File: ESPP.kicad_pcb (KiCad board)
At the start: 2 copper layers, 18 parts, among them P1 USB_OTG, Q1 MMBT3904, Q2 MMBT3904, U1 RT9193, U2 CH340G, X1 12MHz, X2 ESP-PROG

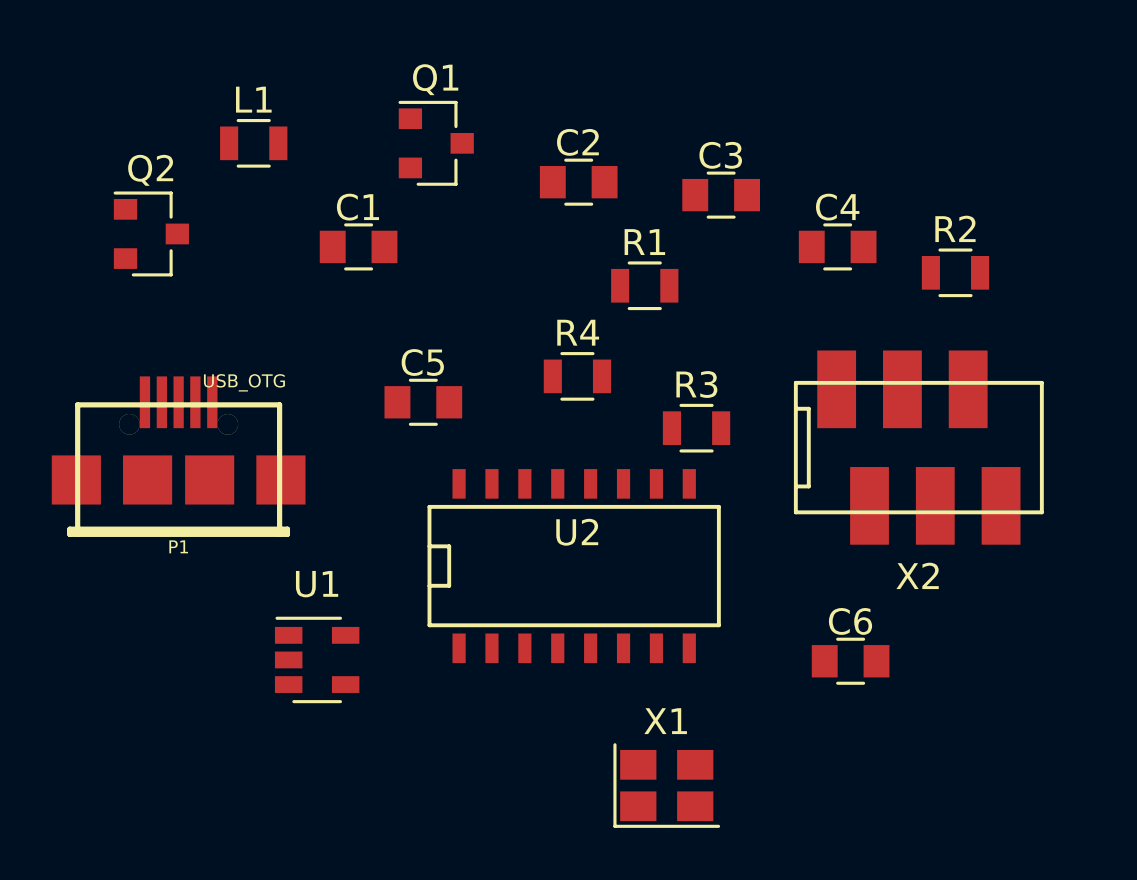
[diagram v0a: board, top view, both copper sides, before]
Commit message: WIP
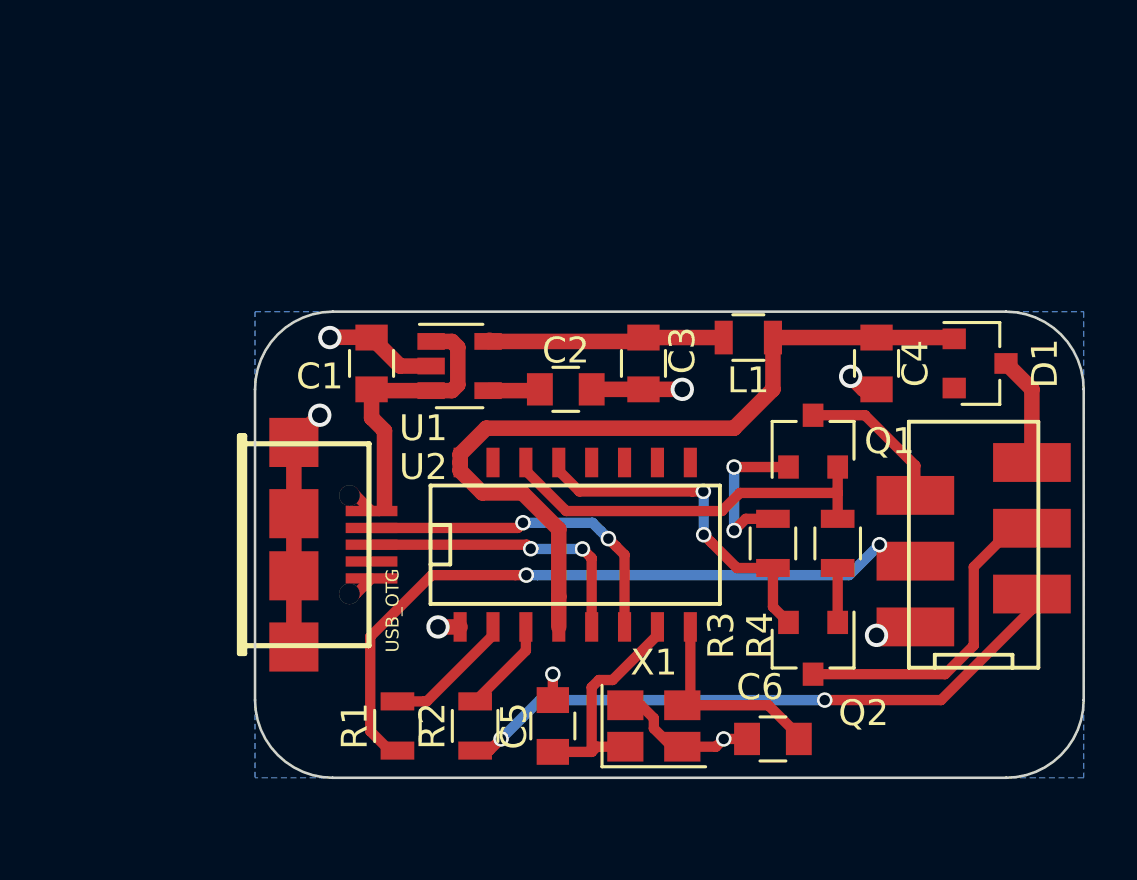
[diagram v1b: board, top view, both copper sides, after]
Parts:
- added D1: BAT54C, TO_SOT_Packages_SMD:SOT-23, F.Cu at (163.0, 105.0)
- added REF***: OSHW-Logo_11.4x12mm_SilkScreen, Symbols:OSHW-Logo_11.4x12mm_SilkScreen, B.Cu at (152.5, 112.0)
- C3: value 47u -> 1u
- moved Q2 30.1 mm to (156.6, 116.0), turned to 270 degrees
- moved R2 25.5 mm to (143.5, 119.0), turned to 90 degrees
- moved L1 20.5 mm to (154.1, 104.0), turned to 180 degrees
- moved R1 19.5 mm to (140.5, 119.0), turned to 90 degrees
- moved Q1 18.5 mm to (156.6, 108.0), turned to 90 degrees
- moved C5 13.5 mm to (146.5, 119.0), turned to 90 degrees
- moved U1 12.6 mm to (142.9, 105.1)
- moved R4 11.9 mm to (157.5, 112.0), turned to 90 degrees
- moved C2 8.02 mm to (147.0, 106.0)
- moved C3 7.16 mm to (150.0, 105.0), turned to 270 degrees
- moved R3 5.34 mm to (155.0, 112.0), turned to 90 degrees
- moved P1 5.10 mm to (136.5, 112.0), turned to 270 degrees
- moved C4 4.74 mm to (159.0, 105.0), turned to 270 degrees
- moved C1 4.53 mm to (139.5, 105.0), turned to 90 degrees
- moved X2 4.31 mm to (162.8, 112.0), turned to 90 degrees
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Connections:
- net /5V renamed /5V-USB
- X2 pad 6: VCC -> Net-(D1-Pad3)
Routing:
- net VCC: track 0.00 -> 31.3 mm
- net GND: track 0.00 -> 28.9 mm, vias 0 -> 8
- net /RX: track 0.00 -> 28.3 mm, vias 0 -> 2
- net /TX: track 0.00 -> 24.3 mm, vias 0 -> 2
- net /RTS: track 0.00 -> 15.3 mm
- net /DTR: track 0.00 -> 13.5 mm, vias 0 -> 2
- net /D-: track 0.00 -> 13.2 mm, vias 0 -> 2
- net /GPIO0: track 0.00 -> 12.6 mm
- net /5V-USB: track 0.00 -> 12.4 mm
- net /D+: track 0.00 -> 11.4 mm, vias 0 -> 2
- net Net-(C3-Pad1): track 0.00 -> 9.23 mm
- net Net-(C5-Pad1): track 0.00 -> 9.07 mm
- net Net-(C6-Pad1): track 0.00 -> 8.27 mm
- net Net-(Q1-Pad1): track 0.00 -> 6.24 mm, vias 0 -> 2
- net /RESET: track 0.00 -> 5.91 mm
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- added copper zone on B.Cu, net GND
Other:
- board outline added: 32 x 18 mm
- board text added: "CC-BY-SA"
- board text added: "DEVICE.FARM"
- board text added: "ESPP 1.0"
